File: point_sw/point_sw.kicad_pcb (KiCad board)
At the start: 2 copper layers, 50.5 x 67.5 mm, 16 parts, among them sw01 C_Radial_D16.0mm_H31.5mm_P7.5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

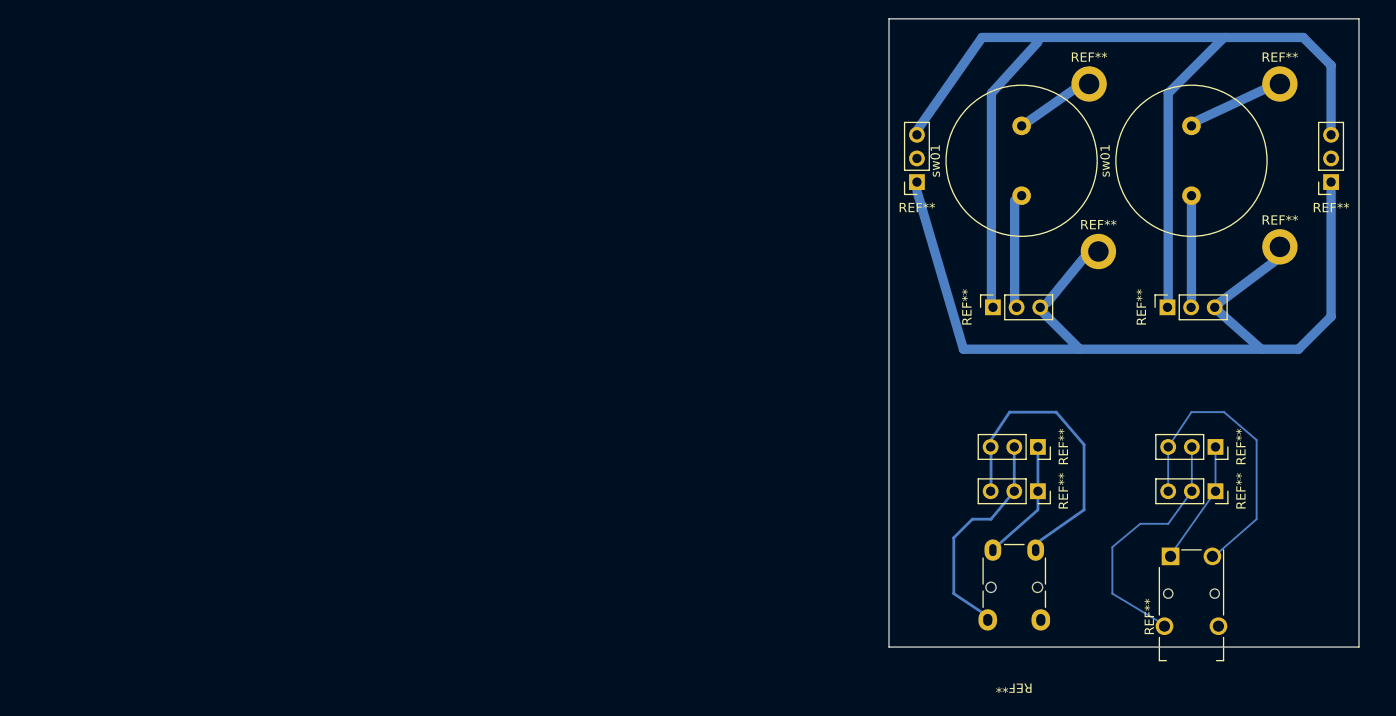
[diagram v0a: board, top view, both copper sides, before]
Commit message: 未来祭用の即席量産
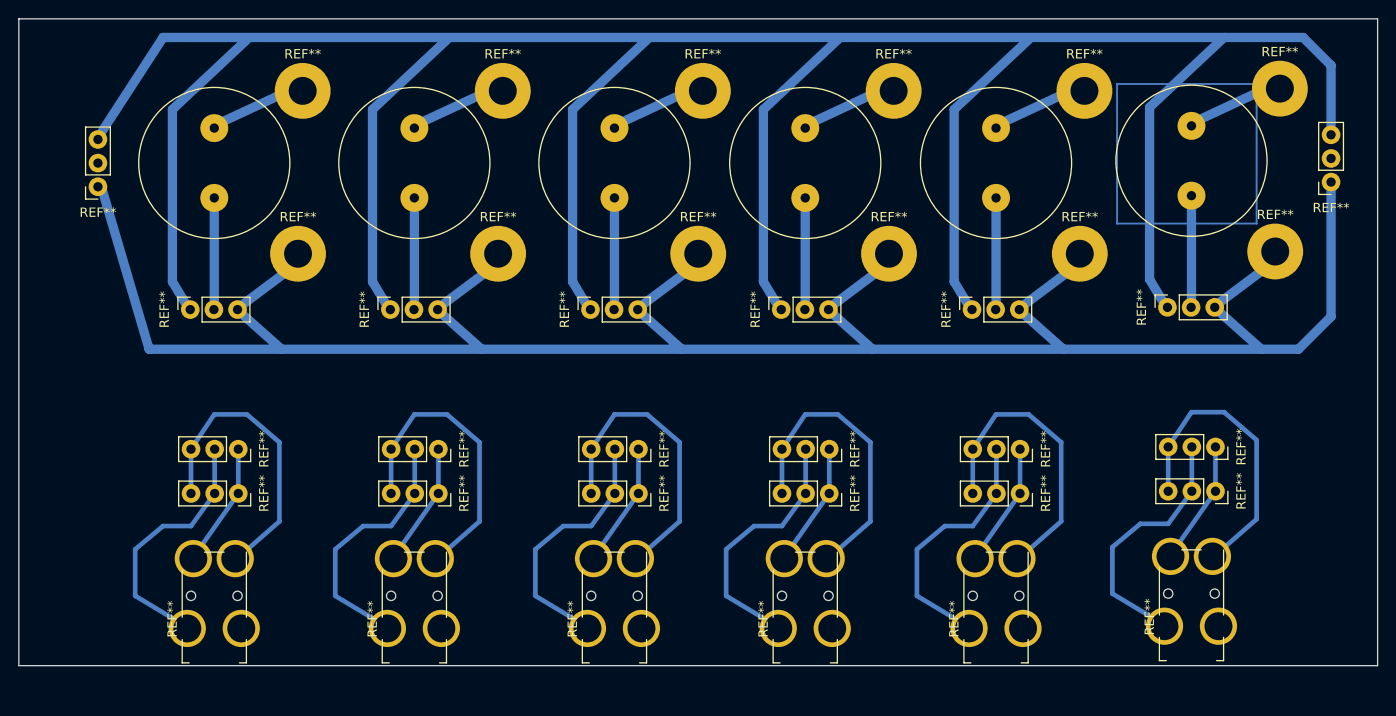
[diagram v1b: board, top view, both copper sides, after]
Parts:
- removed the REF** at (199.5, 85.5)
- removed the REF** at (179.0, 68.0)
- removed the REF** at (180.0, 86.0)
- removed the REF** at (173.5, 107.0)
- removed the REF** at (168.7, 92.0)
- removed the REF** at (173.8, 125.6)
- removed the REF** at (199.5, 68.0)
- removed the REF** at (173.5, 111.8)
- removed the sw01 at (171.8, 80.0)
- added REF**: MountingHole_3mm_Pad, MountingHole:MountingHole_3mm_Pad, F.Cu at (178.5, 68.7)
- added REF**: PinSocket_1x03_P2.54mm_Vertical, Connector_PinSocket_2.54mm:PinSocket_1x03_P2.54mm_Vertical, F.Cu at (103.9, 92.2)
- added REF**: MountingHole_3mm_Pad, MountingHole:MountingHole_3mm_Pad, F.Cu at (178.0, 86.2)
- added REF**: PinSocket_1x03_P2.54mm_Vertical, Connector_PinSocket_2.54mm:PinSocket_1x03_P2.54mm_Vertical, F.Cu at (125.4, 92.2)
- added REF**: PinSocket_1x03_P2.54mm_Vertical, Connector_PinSocket_2.54mm:PinSocket_1x03_P2.54mm_Vertical, F.Cu at (87.6, 112.0)
- added REF**: PinSocket_1x03_P2.54mm_Vertical, Connector_PinSocket_2.54mm:PinSocket_1x03_P2.54mm_Vertical, F.Cu at (130.6, 107.2)
- added REF**: PinSocket_1x03_P2.54mm_Vertical, Connector_PinSocket_2.54mm:PinSocket_1x03_P2.54mm_Vertical, F.Cu at (82.4, 92.2)
- added REF**: MountingHole_3mm_Pad, MountingHole:MountingHole_3mm_Pad, F.Cu at (157.5, 86.2)
- added REF**: Jack_3.5mm_Switronic_ST-005-G_horizontal, Connector_Audio:Jack_3.5mm_Switronic_ST-005-G_horizontal, F.Cu at (128.0, 125.5)
- added REF**: PinSocket_1x03_P2.54mm_Vertical, Connector_PinSocket_2.54mm:PinSocket_1x03_P2.54mm_Vertical, F.Cu at (151.1, 107.2)
- added REF**: Jack_3.5mm_Switronic_ST-005-G_horizontal, Connector_Audio:Jack_3.5mm_Switronic_ST-005-G_horizontal, F.Cu at (85.0, 125.5)
- added REF**: PinSocket_1x03_P2.54mm_Vertical, Connector_PinSocket_2.54mm:PinSocket_1x03_P2.54mm_Vertical, F.Cu at (145.9, 92.2)
- added REF**: Jack_3.5mm_Switronic_ST-005-G_horizontal, Connector_Audio:Jack_3.5mm_Switronic_ST-005-G_horizontal, F.Cu at (148.5, 125.5)
- added REF**: MountingHole_3mm_Pad, MountingHole:MountingHole_3mm_Pad, F.Cu at (115.5, 86.2)
- added REF**: MountingHole_3mm_Pad, MountingHole:MountingHole_3mm_Pad, F.Cu at (158.0, 68.7)
- added REF**: MountingHole_3mm_Pad, MountingHole:MountingHole_3mm_Pad, F.Cu at (137.5, 68.7)
- added REF**: MountingHole_3mm_Pad, MountingHole:MountingHole_3mm_Pad, F.Cu at (94.0, 86.2)
- added REF**: PinSocket_1x03_P2.54mm_Vertical, Connector_PinSocket_2.54mm:PinSocket_1x03_P2.54mm_Vertical, F.Cu at (130.6, 112.0)
- added REF**: MountingHole_3mm_Pad, MountingHole:MountingHole_3mm_Pad, F.Cu at (199.0, 86.0)
- added REF**: PinSocket_1x03_P2.54mm_Vertical, Connector_PinSocket_2.54mm:PinSocket_1x03_P2.54mm_Vertical, F.Cu at (171.6, 112.0)
- added REF**: PinSocket_1x03_P2.54mm_Vertical, Connector_PinSocket_2.54mm:PinSocket_1x03_P2.54mm_Vertical, F.Cu at (151.1, 112.0)
- added REF**: MountingHole_3mm_Pad, MountingHole:MountingHole_3mm_Pad, F.Cu at (94.5, 68.7)
- added REF**: MountingHole_3mm_Pad, MountingHole:MountingHole_3mm_Pad, F.Cu at (199.5, 68.5)
- added REF**: PinSocket_1x03_P2.54mm_Vertical, Connector_PinSocket_2.54mm:PinSocket_1x03_P2.54mm_Vertical, F.Cu at (109.1, 112.0)
- added REF**: Jack_3.5mm_Switronic_ST-005-G_horizontal, Connector_Audio:Jack_3.5mm_Switronic_ST-005-G_horizontal, F.Cu at (169.0, 125.5)
- added REF**: PinSocket_1x03_P2.54mm_Vertical, Connector_PinSocket_2.54mm:PinSocket_1x03_P2.54mm_Vertical, F.Cu at (171.6, 107.2)
- added REF**: PinSocket_1x03_P2.54mm_Vertical, Connector_PinSocket_2.54mm:PinSocket_1x03_P2.54mm_Vertical, F.Cu at (109.1, 107.2)
- added REF**: MountingHole_3mm_Pad, MountingHole:MountingHole_3mm_Pad, F.Cu at (137.0, 86.2)
- added REF**: PinSocket_1x03_P2.54mm_Vertical, Connector_PinSocket_2.54mm:PinSocket_1x03_P2.54mm_Vertical, F.Cu at (87.6, 107.2)
- added REF**: PinSocket_1x03_P2.54mm_Vertical, Connector_PinSocket_2.54mm:PinSocket_1x03_P2.54mm_Vertical, F.Cu at (166.4, 92.2)
- added REF**: MountingHole_3mm_Pad, MountingHole:MountingHole_3mm_Pad, F.Cu at (116.0, 68.7)
- added REF**: Jack_3.5mm_Switronic_ST-005-G_horizontal, Connector_Audio:Jack_3.5mm_Switronic_ST-005-G_horizontal, F.Cu at (106.5, 125.5)
- added sw01: C_Radial_D16.0mm_H31.5mm_P7.50mm, Capacitor_THT:C_Radial_D16.0mm_H31.5mm_P7.50mm, F.Cu at (148.5, 80.2)
- added sw01: C_Radial_D16.0mm_H31.5mm_P7.50mm, Capacitor_THT:C_Radial_D16.0mm_H31.5mm_P7.50mm, F.Cu at (128.0, 80.2)
- added sw01: C_Radial_D16.0mm_H31.5mm_P7.50mm, Capacitor_THT:C_Radial_D16.0mm_H31.5mm_P7.50mm, F.Cu at (169.0, 80.2)
- added sw01: C_Radial_D16.0mm_H31.5mm_P7.50mm, Capacitor_THT:C_Radial_D16.0mm_H31.5mm_P7.50mm, F.Cu at (85.0, 80.2)
- added sw01: C_Radial_D16.0mm_H31.5mm_P7.50mm, Capacitor_THT:C_Radial_D16.0mm_H31.5mm_P7.50mm, F.Cu at (106.5, 80.2)
- moved REF** 88.0 mm to (72.5, 79.0)
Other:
- board size 50.5 x 67.5 mm -> 146 x 69.5 mm
